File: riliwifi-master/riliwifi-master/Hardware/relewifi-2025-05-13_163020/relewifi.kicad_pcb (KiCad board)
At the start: 2 copper layers, 45 parts, among them J10 Screw_Terminal_01x03, J11 Screw_Terminal_01x03, J3 Screw_Terminal_01x03, J4 Screw_Terminal_01x03, J5 Screw_Terminal_01x02, J6 Screw_Terminal_01x03, J7 Screw_Terminal_01x03, J8 Screw_Terminal_01x03, J9 Screw_Terminal_01x03, K1 FINDER-40.52, K2 FINDER-40.52, K3 FINDER-40.52, K4 FINDER-40.52, Q1 Q_NPN_BCE, Q2 Q_NPN_BCE, Q3 Q_NPN_BCE, Q4 Q_NPN_BCE, U1 EL817, U2 EL817, U3 EL817, U4 EL817, U5 L7805, U6 ESP32DevKitv1

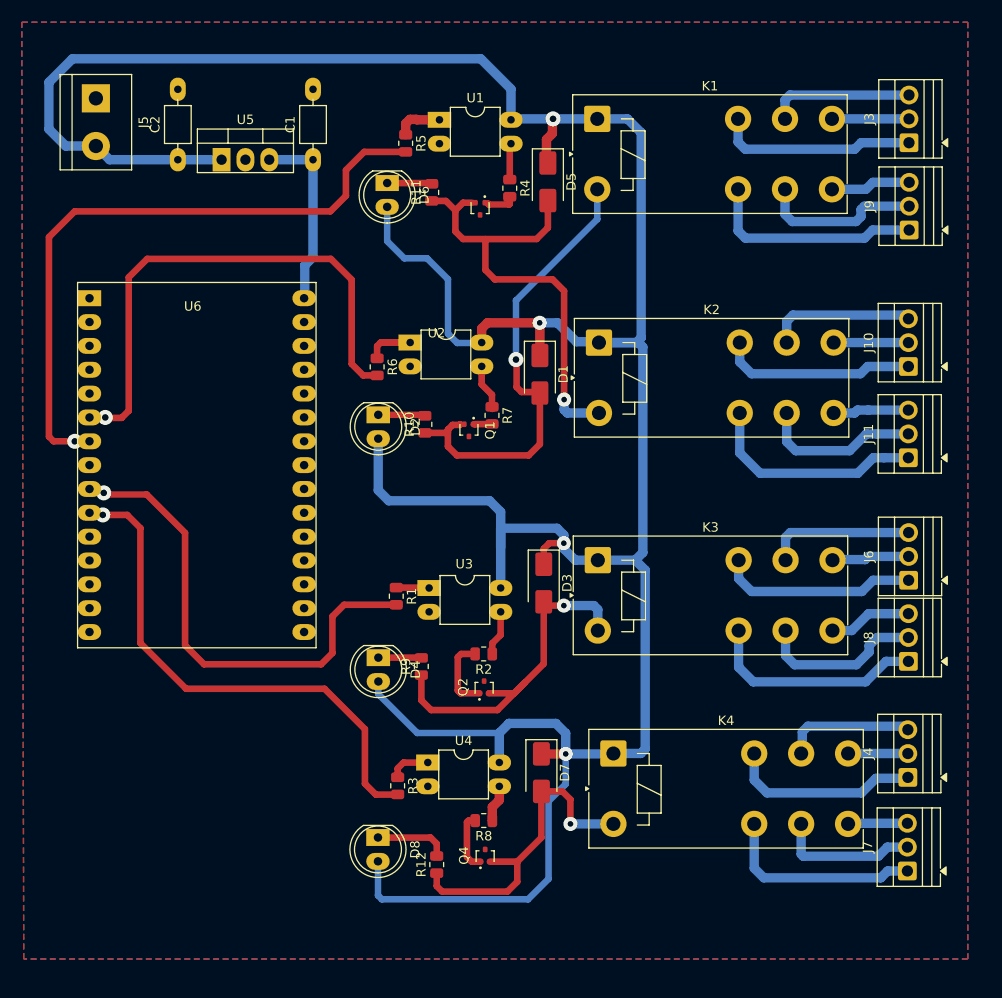
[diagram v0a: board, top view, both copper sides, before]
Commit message: Ultimo Avance PCB
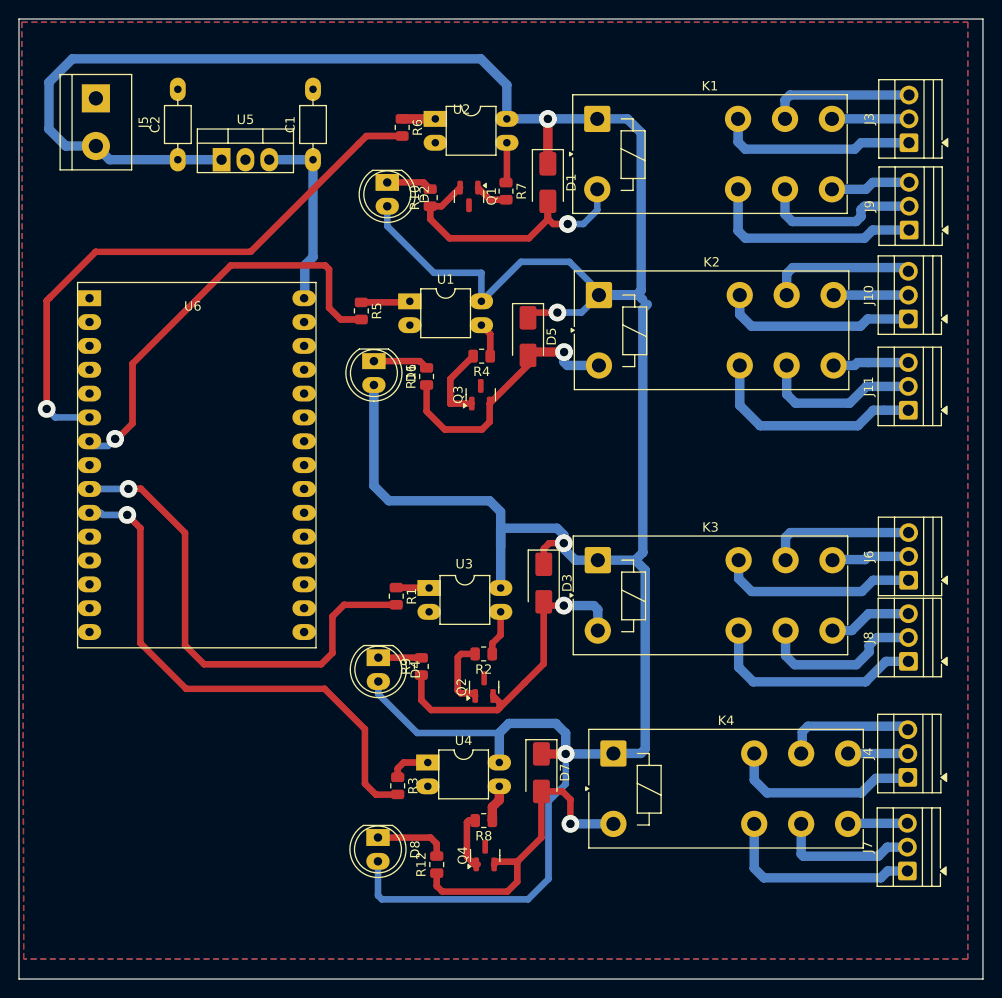
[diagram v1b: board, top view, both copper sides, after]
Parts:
- Q1, Q2, Q3, Q4: footprint Package_TO_SOT_SMD:SOT-416 -> Package_TO_SOT_SMD:SOT-23
- moved R6 25.6 mm to (107.4, 30.1)
- moved Q1 24.9 mm to (114.5, 37.4)
- moved D2 24.8 mm to (105.8, 35.9)
- moved R10 24.2 mm to (110.4, 37.5)
- moved U2 24.0 mm to (110.9, 29.1)
- moved R7 23.9 mm to (118.4, 36.9)
- moved D1 20.4 mm to (122.9, 35.9)
- moved Q3 19.8 mm to (115.7, 58.5), turned to 90 degrees
- moved R11 19.6 mm to (110.0, 56.6)
- moved U1 19.6 mm to (108.2, 48.6)
- moved D6 19.0 mm to (104.4, 55.0)
- moved R5 18.5 mm to (103.0, 49.6)
- moved R4 18.1 mm to (115.8, 54.4), turned to 180 degrees
- moved D5 16.6 mm to (120.8, 52.3)
- moved J11 5.06 mm to (161.3, 60.2)
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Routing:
- net GIOP39: track 69.1 -> 45.7 mm
- net Net-(D5-A): track 50.0 -> 28.4 mm
- net Net-(D1-A): track 49.8 -> 31.7 mm
- net RV-VCC: track 342.4 -> 349.9 mm
- net Net-(Q3-B): track 3.16 -> 8.37 mm
- net GIOP36: track 56.4 -> 61.6 mm
- net Net-(R6-Pad1): track 8.09 -> 3.53 mm
- net Net-(D3-A): track 37.4 -> 34.7 mm
- net Net-(R7-Pad1): track 5.37 -> 3.60 mm
- net Net-(Q1-B): track 1.99 -> 3.53 mm
- net Net-(D6-K): track 4.78 -> 6.05 mm
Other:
- board outline added: 102.7 x 102.3 mm
